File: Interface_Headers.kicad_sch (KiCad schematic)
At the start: 13 parts, among them J1 BTB_10132798-062100LF, J22 USB_C_Receptacle_USB2.0_16P, J3 SWDB, U7 USBLC6-2SC6

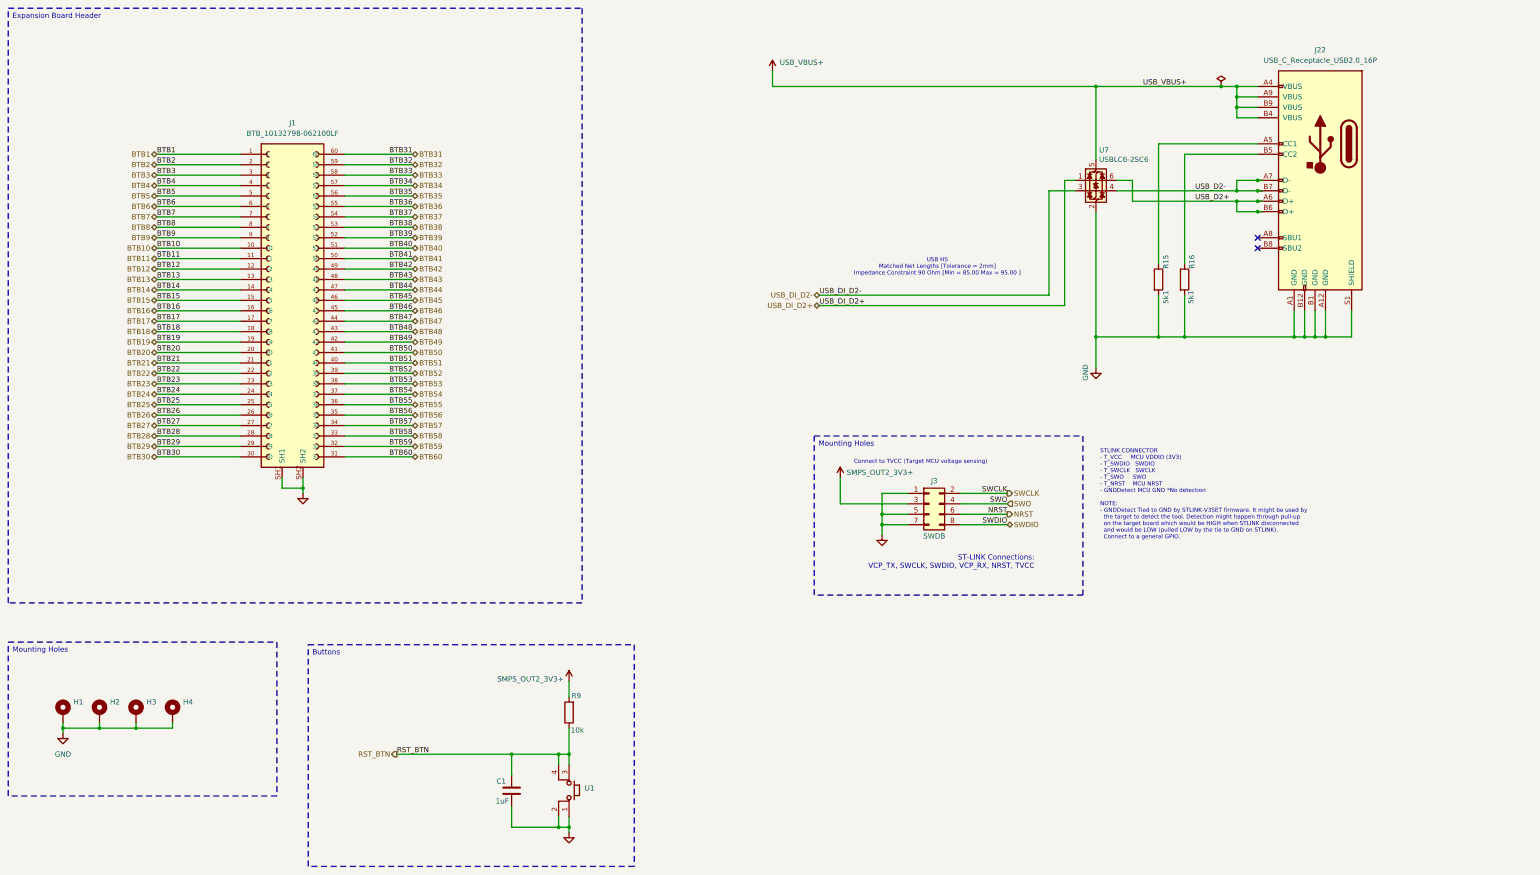
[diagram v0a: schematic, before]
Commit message: Update
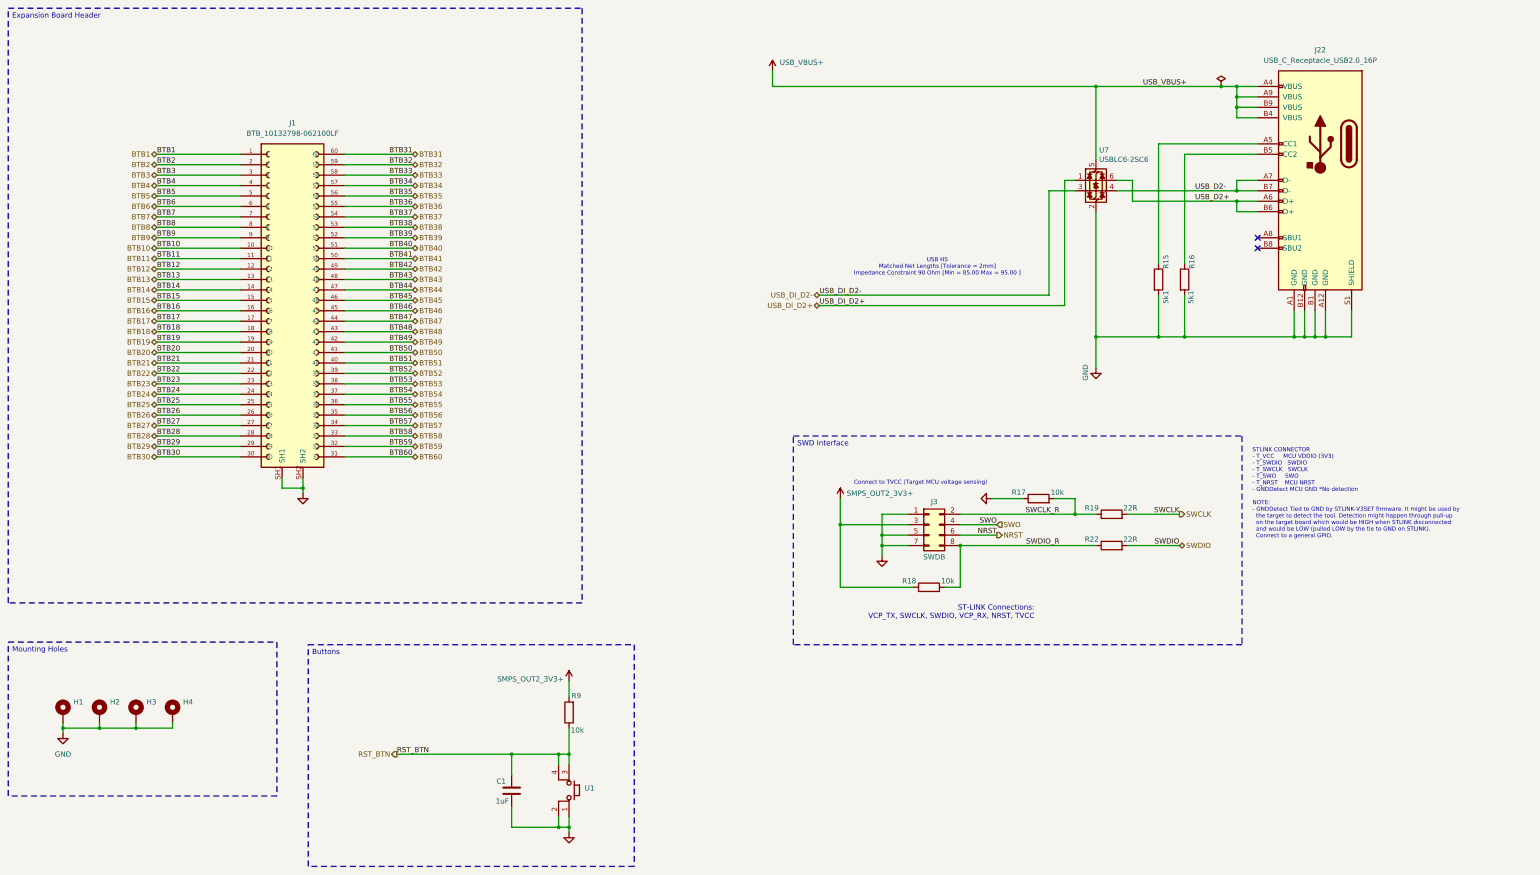
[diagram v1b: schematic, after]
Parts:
- added R17, R18: 10k, Resistor_SMD:R_0603_1608Metric, symbol Device:R
- added R19, R22: 22R, Resistor_SMD:R_0603_1608Metric, symbol Device:R
- U1: value ~ -> (none)
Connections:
- net GND: now also R17.1
- net SMPS_OUT2_3V3+: now also R18.1
- net SWCLK: now also R19.2; no longer J3.2 (Pin_2)
- net SWDIO: now also R22.2; no longer J3.8 (Pin_8)
- new net SWCLK_R: J3.2 (Pin_2), R17.2, R19.1
- new net SWDIO_R: J3.8 (Pin_8), R18.2, R22.1
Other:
- moved on the sheet: J3
